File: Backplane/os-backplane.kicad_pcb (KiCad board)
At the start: 4 copper layers, 195 x 95 mm, 163 parts, among them J1 FPANEL, J2 FAN, J3 PWR, Q1 IRFML8244, Q10 CSD18503Q5A, Q11 MMUN2231L, Q2 AOD4189, Q3 AOD4189, Q4 MMBT3906, Q5 MMBT3904, Q6 MMBT3904, Q7 CSD18504Q5A, Q8 MMUN2231L, Q9 CSD18504Q5A, U1 LM25116MHX, U2 LM25088-1MH

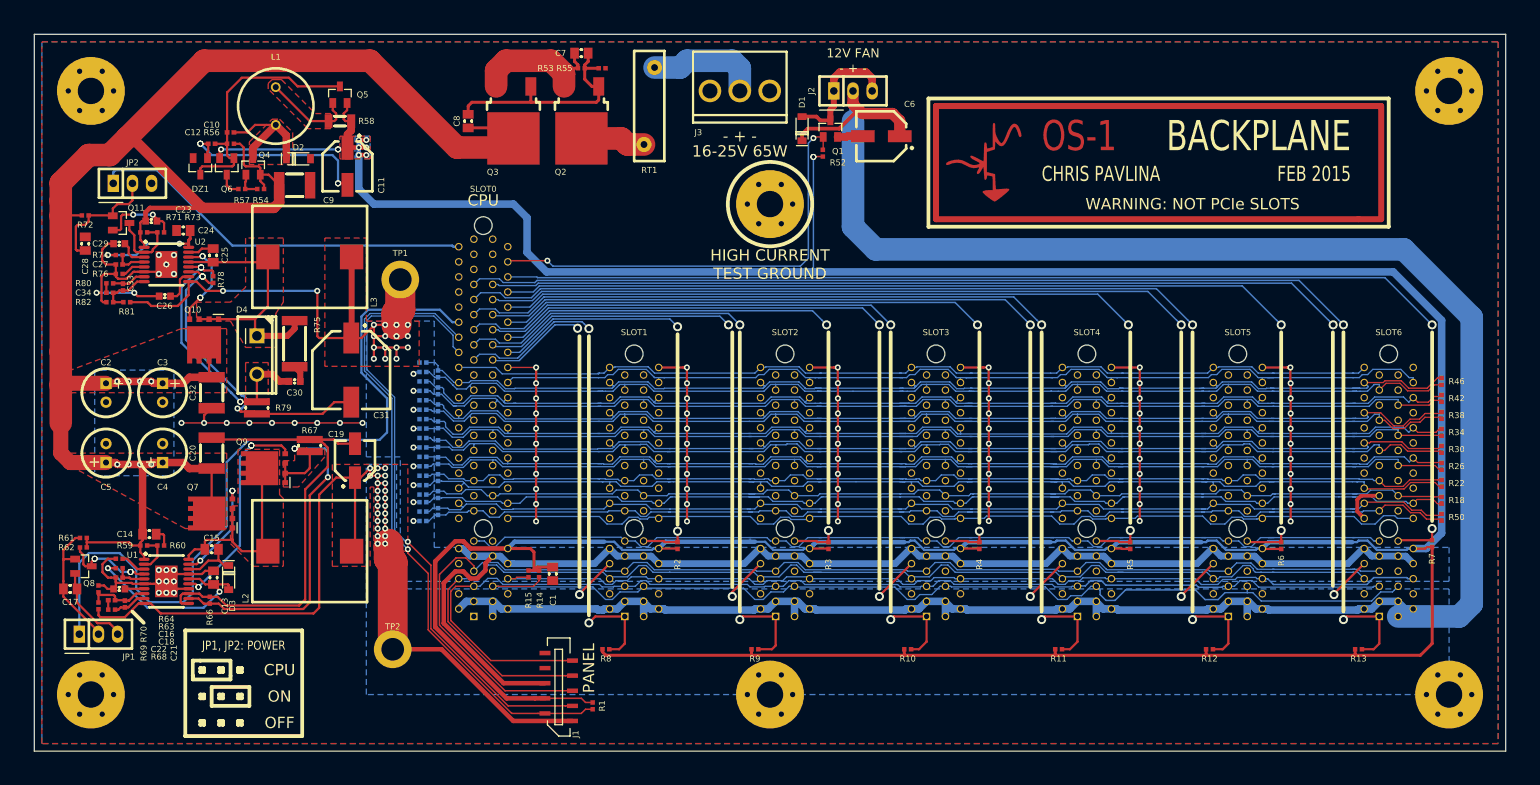
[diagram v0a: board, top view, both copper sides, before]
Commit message: Finished to send to fab
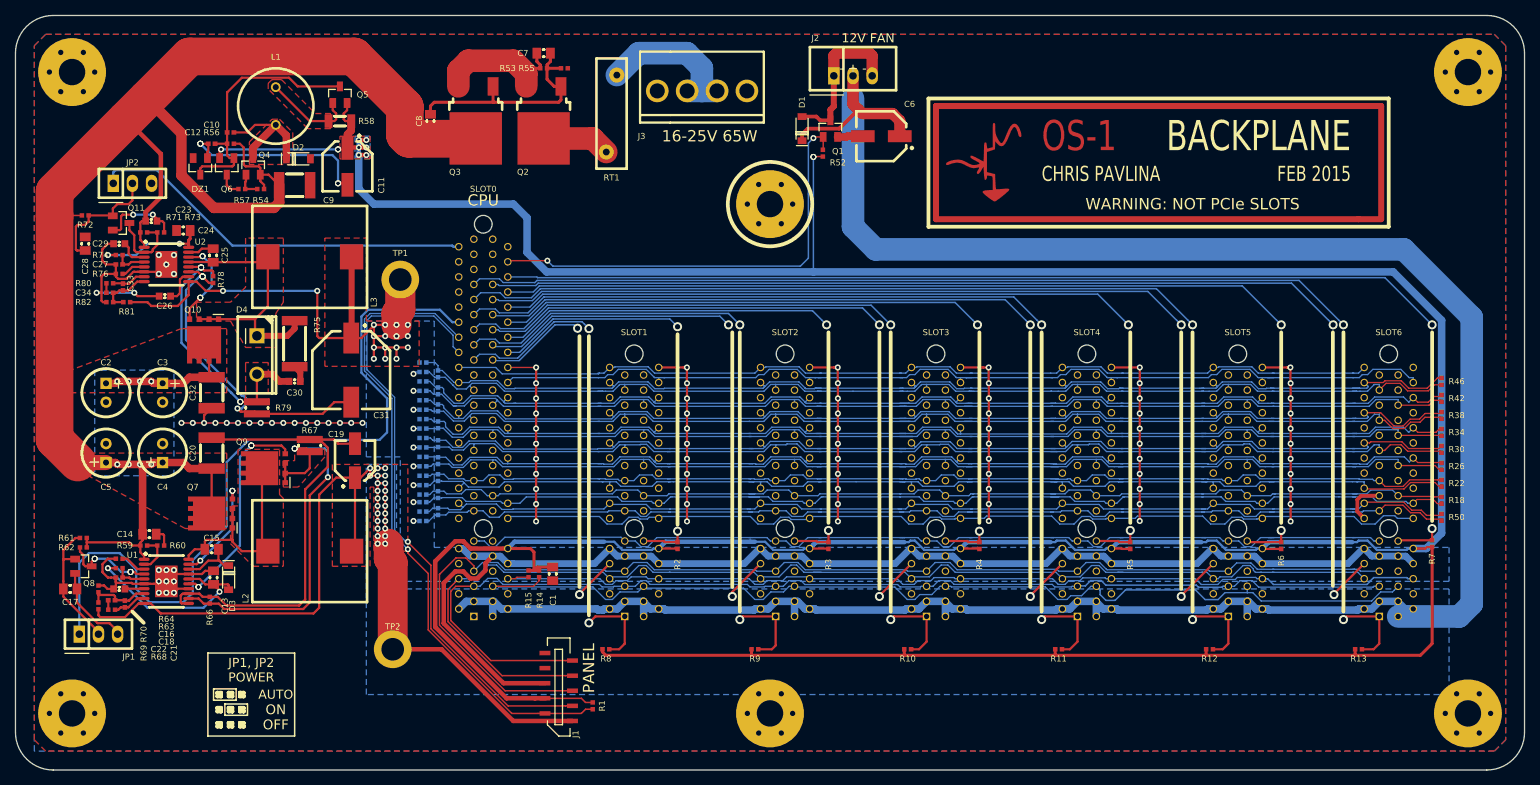
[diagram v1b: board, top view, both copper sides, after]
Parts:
- removed the G*** at (215.0, 77.5)
- added G***1: LOGO, LOGO, B.Cu at (217.5, 75.0)
- J2: footprint conn-100mil:CONN-100MIL-M-1x3 -> conn-100mil:CONN-100MIL-M-1x3-SHROUD
- J3: value PWR -> POWER
- moved RT1 5.10 mm to (104.0, 68.0)
- moved C7 5.00 mm to (95.0, 60.0)
- moved C8 5.00 mm to (80.0, 69.0)
- moved J3 5.00 mm to (116.0, 65.0)
- moved Q2 5.00 mm to (95.0, 68.0)
- moved Q3 5.00 mm to (86.0, 68.0)
- moved R53 5.00 mm to (95.0, 62.0)
- moved R55 5.00 mm to (97.8, 62.0)
- moved MP1 3.54 mm to (32.5, 147.5)
- moved MP2 3.54 mm to (217.5, 147.5)
- moved MP3 3.54 mm to (32.5, 62.5)
- moved MP4 3.54 mm to (217.5, 62.5)
- moved MP6 2.50 mm to (125.0, 147.5)
- moved J2 2.00 mm to (136.0, 63.0)
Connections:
- J3 pad 3: GND -> Net-(J3-Pad2)
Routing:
- net GND: track 309.8 -> 321.8 mm, vias 105 -> 113
- net +12: track 452.2 -> 459.2 mm
- net Net-(J3-Pad2): track 15.1 -> 20.3 mm
- net Net-(D1-Pad2): track 17.2 -> 20.7 mm
- net /Power/Supply12V/VIN: track 264.9 -> 267.9 mm
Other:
- board size 195 x 95 mm -> 200 x 100 mm
- board text added: "AUTO"
- board text added: "JP1, JP2 POWER"
- board text removed: "HIGH CURRENT TEST GROUND"
- board text removed: "JP1, JP2: POWER"
